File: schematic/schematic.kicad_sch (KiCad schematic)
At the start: 20 parts, among them M1 Motor_DC, M2 Motor_DC, M3 Motor_DC, M4 Motor_DC, M5 Motor_Servo, M6 Motor_Servo, U1 TCRT5000, U10 TCRT5000, U11 L298N, U2 TCRT5000, U3 TCRT5000, U4 L298N, U5 LSM9DS1, U6 HC-SR04, U7 HC-SR04, U8 HC-SR04, U9 HC-SR04

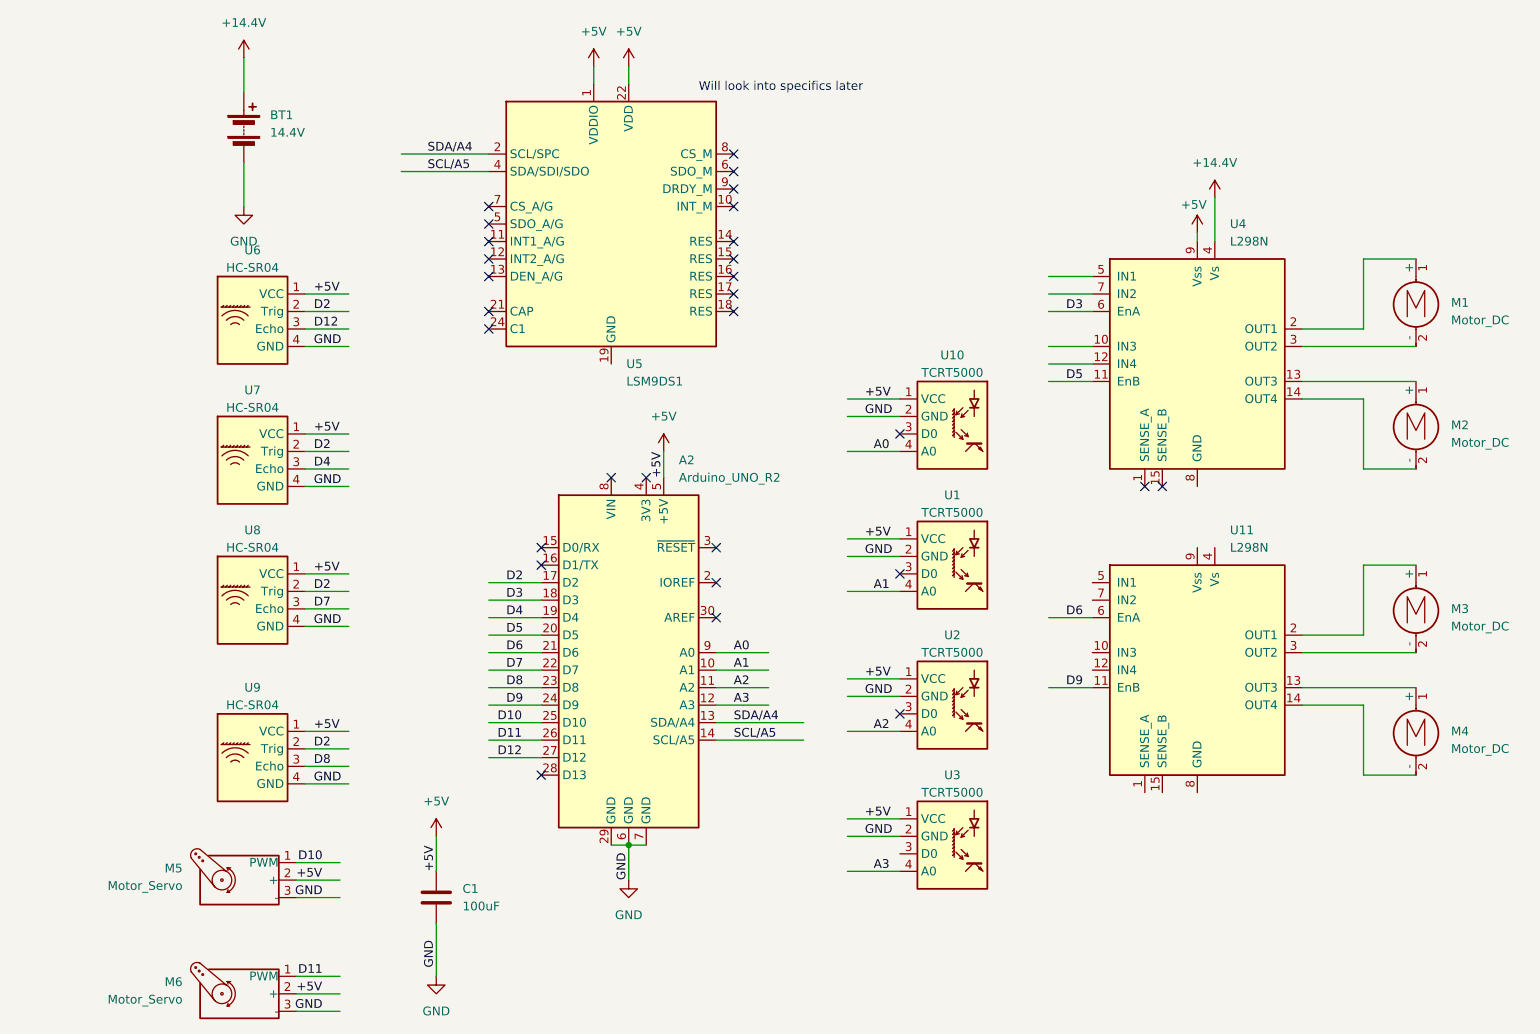
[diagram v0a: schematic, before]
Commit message: schematic updated
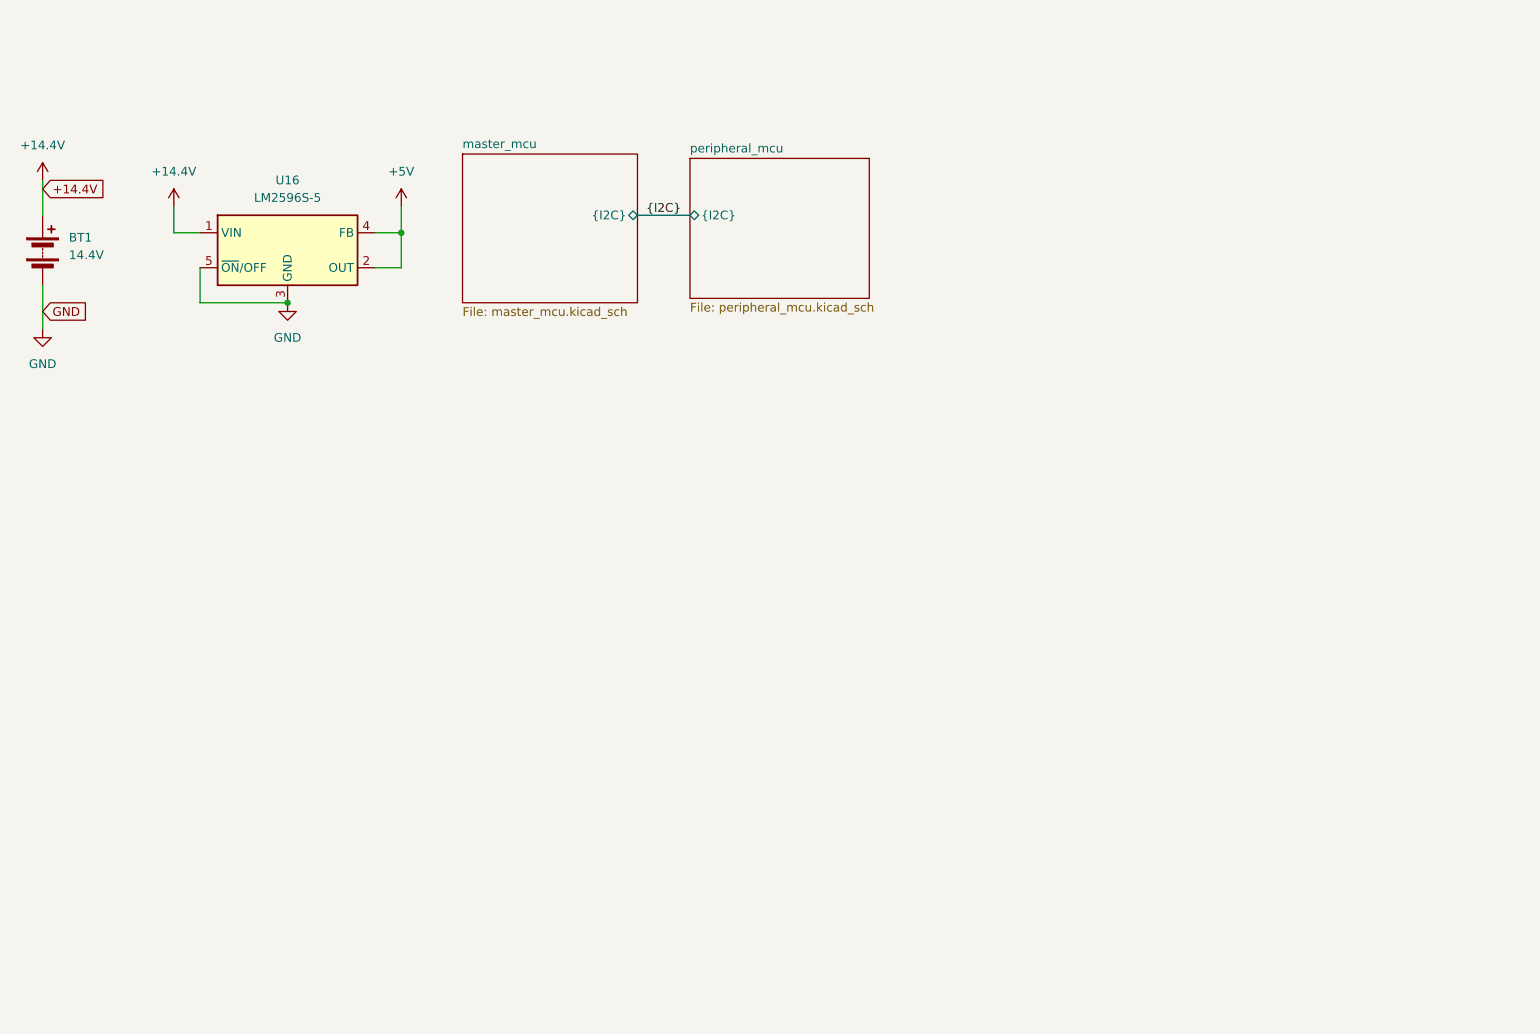
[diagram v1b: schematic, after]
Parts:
- removed A2: Arduino_UNO_R2, Module:Arduino_UNO_R2, symbol MCU_Module:Arduino_UNO_R2
- removed C1: 100uF, symbol Device:C
- removed M1, M2, M3, M4: Motor_DC, symbol Motor:Motor_DC
- removed M5, M6: Motor_Servo, symbol Motor:Motor_Servo
- removed U1, U10, U2, U3: TCRT5000, symbol symbol_lib:TCRT5000
- removed U11, U4: L298N, Package_TO_SOT_THT:TO-220-15_P2.54x2.54mm_StaggerOdd_Lead4.58mm_Vertical, symbol Driver_Motor:L298N
- removed U5: LSM9DS1, Package_LGA:LGA-24L_3x3.5mm_P0.43mm, symbol Sensor_Motion:LSM9DS1
- removed U6, U7, U8, U9: HC-SR04, symbol symbol_lib:HC-SR04
- added U16: LM2596S-5, Package_TO_SOT_SMD:TO-263-5_TabPin3, symbol Regulator_Switching:LM2596S-5
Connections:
- net +14.4V: now also U16.1 (VIN)
- net +5V: now also U16.2 (OUT), U16.4 (FB)
- net GND: now also U16.3 (GND), U16.5 (~{ON}/OFF)
- no-connect marks 29 -> 0
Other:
- added sheet master_mcu (master_mcu.kicad_sch)
- added sheet peripheral_mcu (peripheral_mcu.kicad_sch)
- note removed: "Will look into specifics later"
- moved on the sheet: BT1
